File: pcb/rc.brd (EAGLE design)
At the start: 64.8 x 69.2 mm, 67 parts, among them IC2 TP4056

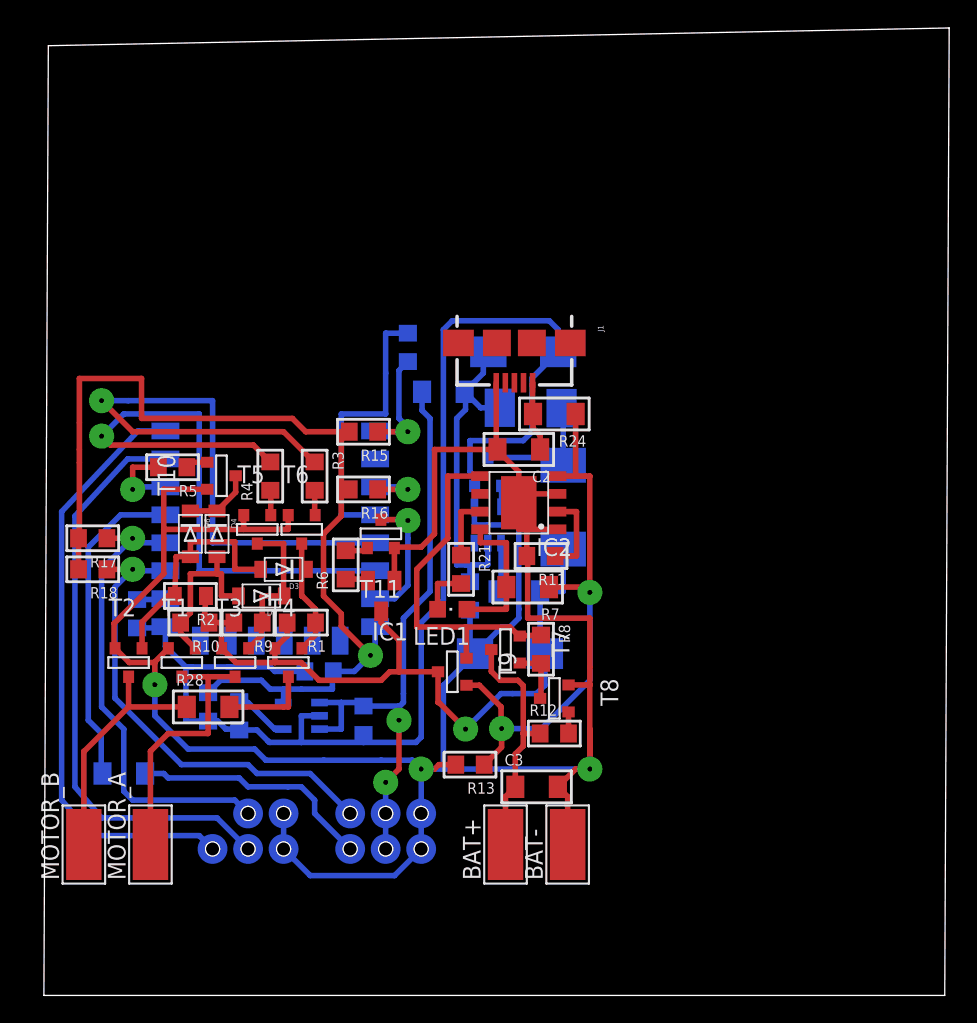
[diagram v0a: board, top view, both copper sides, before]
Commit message: pcb
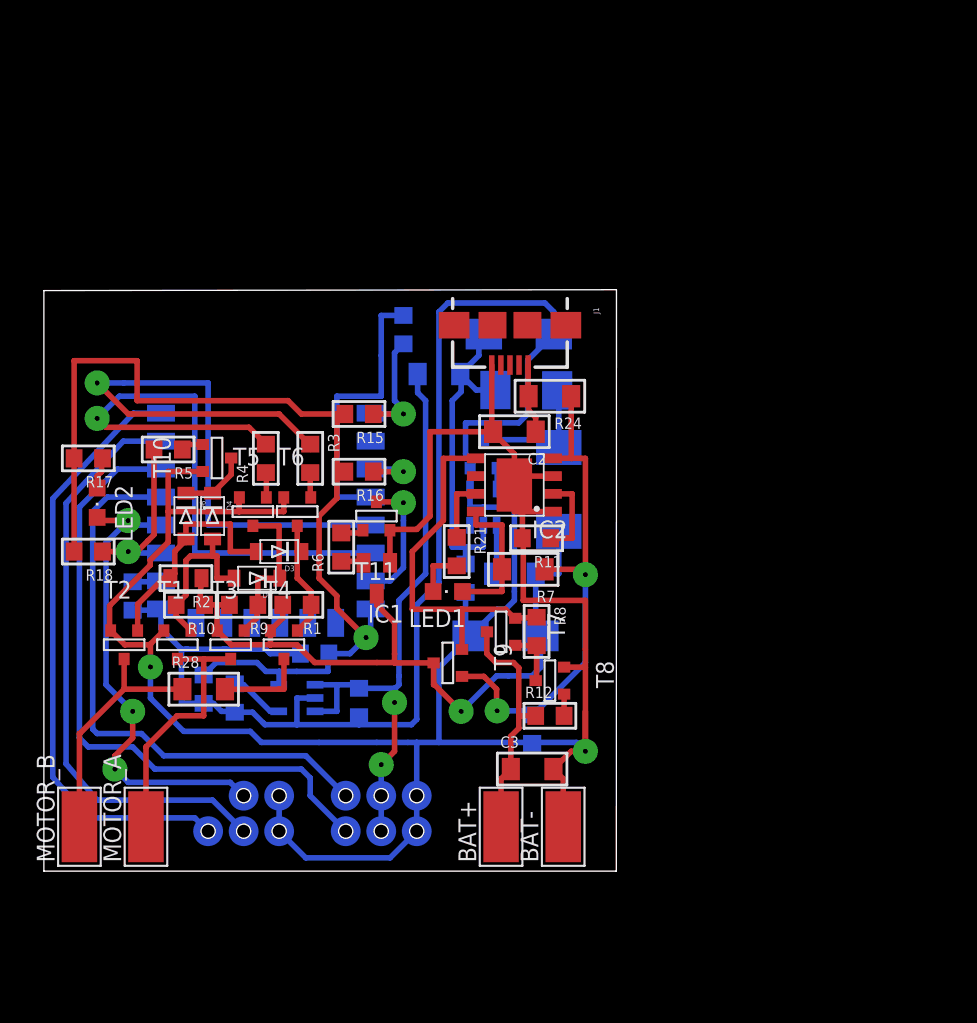
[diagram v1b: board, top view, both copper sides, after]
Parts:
- removed R22: 0, skydrop:R1206
- added LED2: (no value), led:CHIPLED_0805
- moved R17 5.72 mm to (1.27, 33.0)
- moved R13 5.12 mm to (33.0, 13.7), flipped to the bottom, turned to 270 degrees
- moved IC1 1.31 mm to (21.9, 24.4)
- moved R24 1.31 mm to (34.3, 37.5)
- moved R29 1.31 mm to (26.4, 39.1)
- moved T10 1.31 mm to (10.5, 33.0)
- moved C7 1.31 mm to (28.3, 24.4)
- moved D2 1.31 mm to (13.3, 24.4)
- moved J1 1.31 mm to (31.4, 42.5)
- moved R15 1.31 mm to (20.6, 36.2)
- moved R16 1.31 mm to (20.6, 32.1)
- moved R2 1.31 mm to (8.26, 24.4)
- moved R3 1.31 mm to (17.1, 33.0)
- moved R4 1.31 mm to (14.0, 33.0)
- moved R5 1.31 mm to (6.99, 33.7)
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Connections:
- removed net N$22: JP4.1, R22.1
- new net N$24: LED2.A, R17.1
- net H_PWM: now also R18.1, U1.GPIO2; no longer U1.GPIO5
- net N$21: now also LED2.C; no longer R17.1
- net SERVO#1_CTRL: now also JP1.1; no longer R22.2
- net SERVO#2_CTRL: now also JP4.1, U1.GPIO5; no longer JP1.1, R18.1, U1.GPIO2
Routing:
- net SERVO#1_CTRL: track 23.1 -> 40.9 mm
- net N$22: track 17.5 -> 0.00 mm
- net SERVO#2_CTRL: track 34.3 -> 46.0 mm, vias 1 -> 0
- net H_PWM: track 5.85 -> 12.7 mm
- net GND: track 285.8 -> 282.2 mm, vias 3 -> 2
- net V_CHRG: track 40.7 -> 37.6 mm
- net N$24: track 0.00 -> 2.28 mm
- net N$21: track 34.5 -> 35.5 mm, vias 1 -> 3
- net BAT_CHRG: track 25.5 -> 26.1 mm
- net N$36: track 19.2 -> 18.7 mm
- net N$9: track 17.3 -> 16.7 mm
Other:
- board size 64.8 x 69.2 mm -> 41 x 41.6 mm
